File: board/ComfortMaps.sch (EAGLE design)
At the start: 47 parts, among them J1 PROG_HDR, J5 0545482271, J6 0545482271, U1 ADXL362, U3 ADP160-3.3, U4 MCP73833, X1 RASPI_GPIO_B+#_PIN

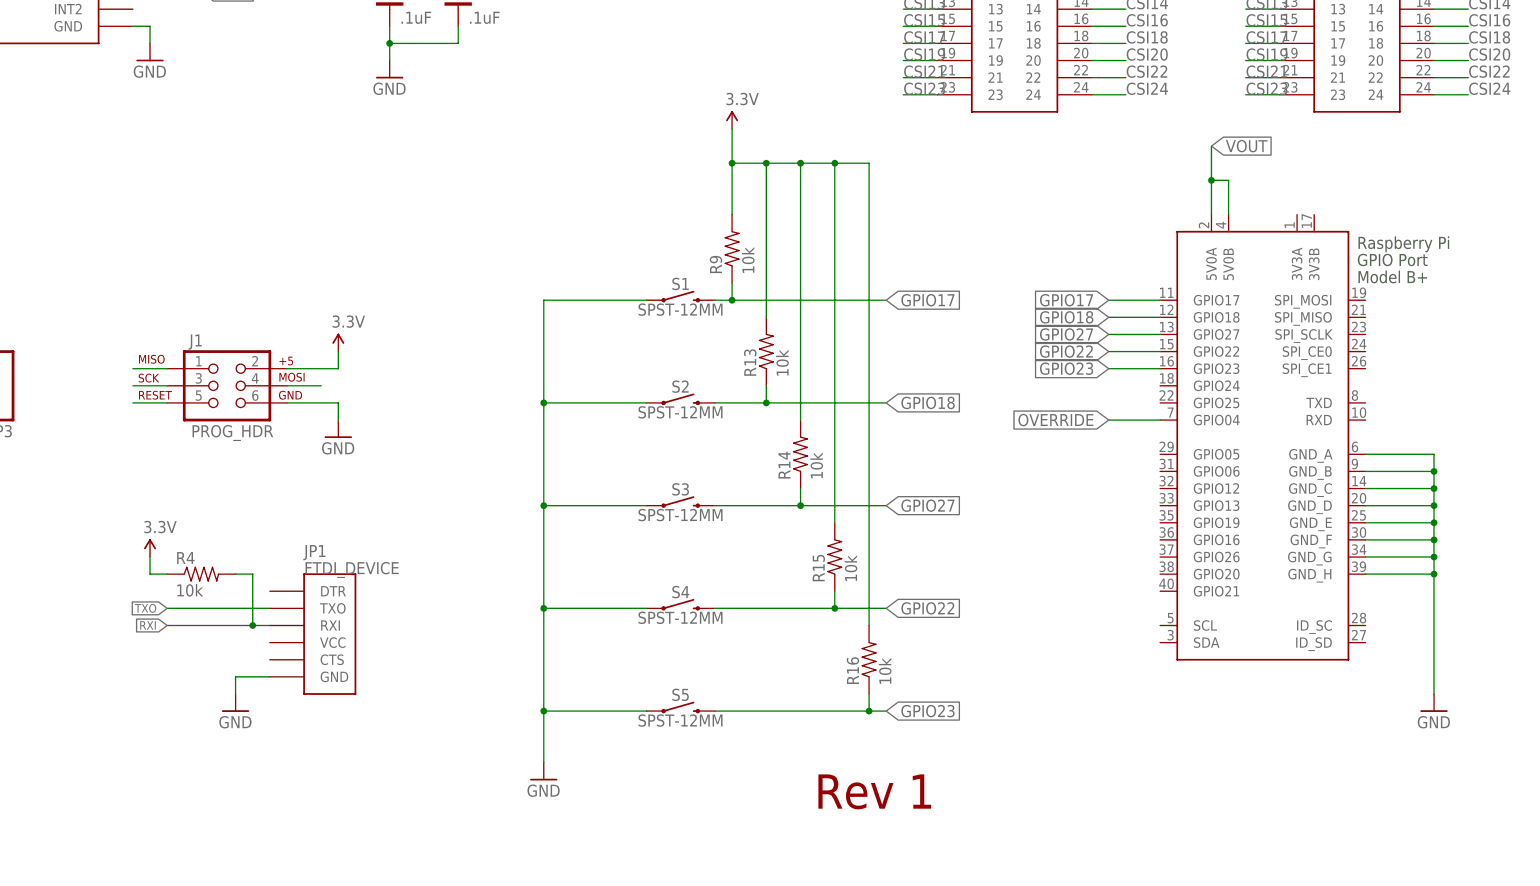
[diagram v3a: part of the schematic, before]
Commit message: Latest, before upwork.
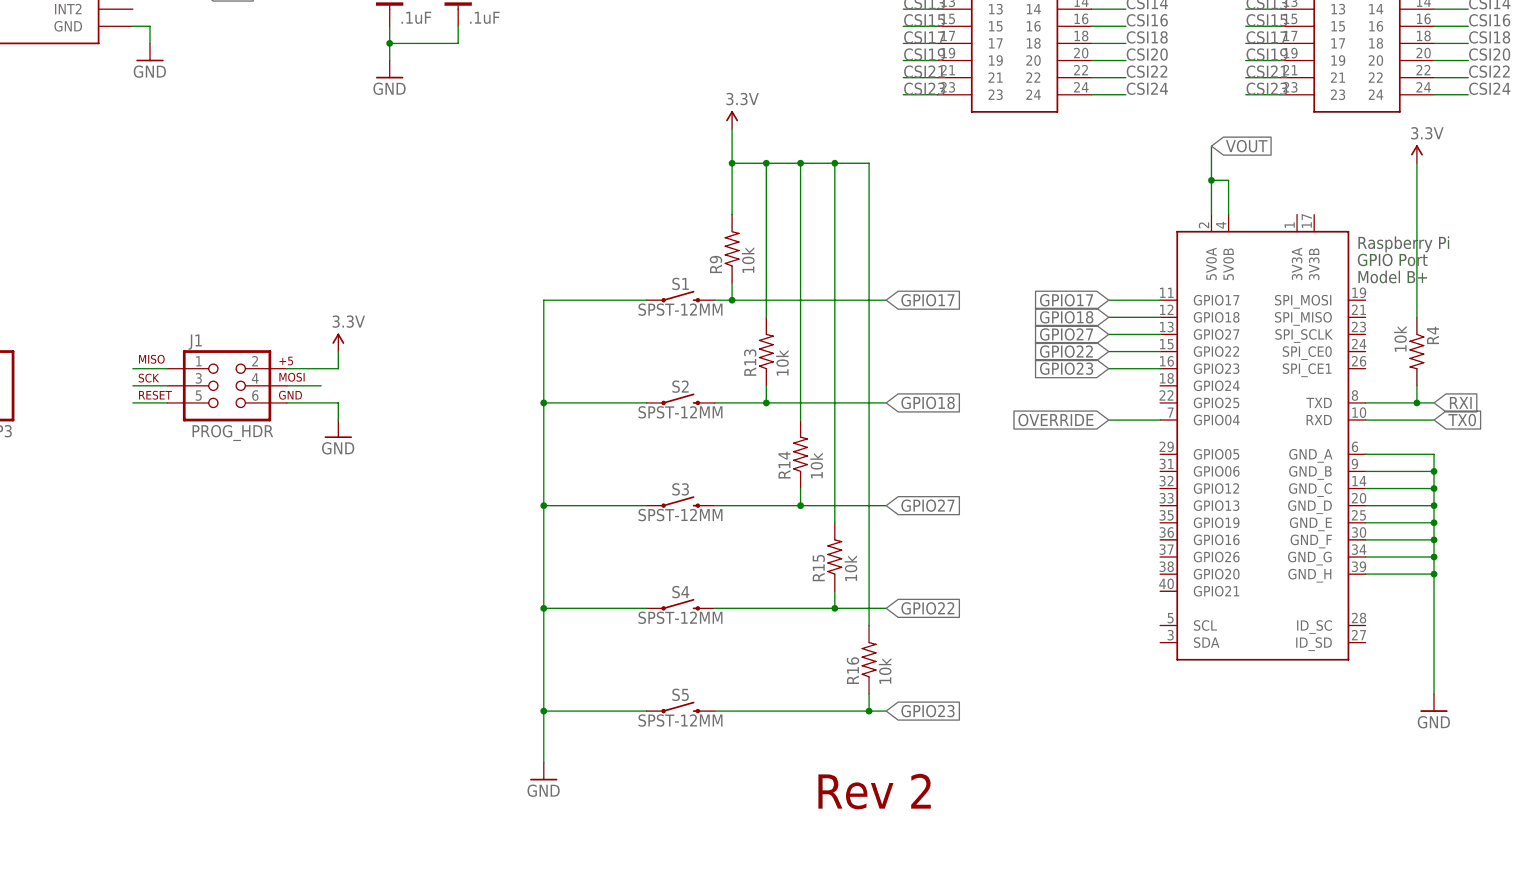
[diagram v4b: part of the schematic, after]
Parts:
- removed JP1: FTDI_DEVICE, SparkFun-Connectors:FTDI_DEVICE
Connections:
- new net TX0: X1.RXD
- net GND: no longer JP1.GND
- net RXI: now also X1.TXD; no longer JP1.RXI
- net TXO: no longer JP1.TXO
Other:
- note added: "Rev 2"
- note removed: "Rev 1"
- moved on the sheet: R4
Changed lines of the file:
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@@
 <?xml version="1.0" encoding="utf-8"?>
 <!DOCTYPE eagle SYSTEM "eagle.dtd">
-<eagle version="9.5.1">
+<eagle version="9.5.2">
 <drawing>
 <settings>
@@
 </part>
 <part name="JP3" library="SparkFun-Connectors" deviceset="M03" device="PTH"/>
-<part name="JP1" library="SparkFun-Connectors" deviceset="FTDI_DEVICE" device=""/>
 <part name="D2" library="SparkFun-DiscreteSemi" deviceset="DIODE-SCHOTTKY" device="" value="RB751">
 <attribute name="PROD_ID" value="DIO-11018"/>
@@
 </part>
 <part name="P+6" library="SparkFun-Aesthetics" deviceset="3.3V" device=""/>
-<part name="GND7" library="SparkFun-Aesthetics" deviceset="GND" device=""/>
 <part name="R4" library="SparkFun-Resistors" deviceset="10K-1%" device="RES-00824" value="10k">
 <attribute name="PROD_ID" value="RES-00824"/>
@@
 <sheet>
 <plain>
-<text x="238.252" y="5.842" size="5.08" layer="94">Rev 1</text>
+<text x="238.252" y="5.842" size="5.08" layer="94">Rev 2</text>
 <text x="2.54" y="2.54" size="1.778" layer="94">Original wake-on-shake concept by
 Nitzan Gadish, Analog Devices</text>
@@
 <attribute name="NAME" x="119.38" y="62.738" size="1.778" layer="95" rot="R180"/>
 </instance>
-<instance part="JP1" gate="G$1" x="162.56" y="33.02" smashed="yes">
-<attribute name="NAME" x="162.56" y="43.18" size="1.778" layer="95"/>
-<attribute name="VALUE" x="162.56" y="40.64" size="1.778" layer="96"/>
-</instance>
 <instance part="D2" gate="G$1" x="66.04" y="45.72" smashed="yes">
 <attribute name="PROD_ID" x="66.04" y="45.72" size="1.778" layer="96" display="off"/>
@@
 <attribute name="VALUE" x="16.764" y="140.716" size="1.778" layer="96"/>
 </instance>
-<instance part="GND7" gate="1" x="152.4" y="20.32" smashed="yes">
-<attribute name="VALUE" x="149.86" y="17.78" size="1.778" layer="96"/>
-</instance>
-<instance part="R4" gate="G$1" x="147.32" y="40.64" smashed="yes">
-<attribute name="PROD_ID" x="147.32" y="40.64" size="1.778" layer="96" display="off"/>
-<attribute name="NAME" x="143.51" y="42.1386" size="1.778" layer="95"/>
-<attribute name="VALUE" x="143.51" y="37.338" size="1.778" layer="96"/>
-</instance>
-<instance part="P+7" gate="G$1" x="139.7" y="43.18" smashed="yes">
-<attribute name="VALUE" x="138.684" y="46.736" size="1.778" layer="96"/>
+<instance part="R4" gate="G$1" x="327.66" y="73.66" smashed="yes" rot="R270">
+<attribute name="PROD_ID" x="327.66" y="73.66" size="1.778" layer="96" rot="R270" display="off"/>
+<attribute name="NAME" x="329.1586" y="77.47" size="1.778" layer="95" rot="R270"/>
+<attribute name="VALUE" x="324.358" y="77.47" size="1.778" layer="96" rot="R270"/>
+</instance>
+<instance part="P+7" gate="G$1" x="327.66" y="101.6" smashed="yes">
+<attribute name="VALUE" x="326.644" y="105.156" size="1.778" layer="96"/>
 </instance>
 <instance part="S1" gate="G$1" x="218.44" y="81.28" smashed="yes">
@@
 <pinref part="GND6" gate="1" pin="GND"/>
 <wire x1="167.64" y1="66.04" x2="167.64" y2="63.5" width="0.1524" layer="91"/>
-</segment>
-<segment>
-<pinref part="JP1" gate="G$1" pin="GND"/>
-<wire x1="157.48" y1="25.4" x2="152.4" y2="25.4" width="0.1524" layer="91"/>
-<wire x1="152.4" y1="25.4" x2="152.4" y2="22.86" width="0.1524" layer="91"/>
-<pinref part="GND7" gate="1" pin="GND"/>
 </segment>
 <segment>
@@
 <segment>
 <pinref part="P+7" gate="G$1" pin="3.3V"/>
-<wire x1="139.7" y1="43.18" x2="139.7" y2="40.64" width="0.1524" layer="91"/>
+<wire x1="327.66" y1="101.6" x2="327.66" y2="78.74" width="0.1524" layer="91"/>
 <pinref part="R4" gate="G$1" pin="1"/>
-<wire x1="139.7" y1="40.64" x2="142.24" y2="40.64" width="0.1524" layer="91"/>
 </segment>
 <segment>
@@
 </segment>
 <segment>
-<pinref part="JP1" gate="G$1" pin="RXI"/>
-<wire x1="157.48" y1="33.02" x2="154.94" y2="33.02" width="0.1524" layer="91"/>
-<label x="142.24" y="33.02" size="1.27" layer="95" rot="R180" xref="yes"/>
+<pinref part="X1" gate="G$1" pin="TXD"/>
+<wire x1="320.04" y1="66.04" x2="327.66" y2="66.04" width="0.1524" layer="91"/>
+<label x="330.2" y="66.04" size="1.778" layer="95" xref="yes"/>
 <pinref part="R4" gate="G$1" pin="2"/>
-<wire x1="154.94" y1="33.02" x2="142.24" y2="33.02" width="0.1524" layer="91"/>
-<wire x1="152.4" y1="40.64" x2="154.94" y2="40.64" width="0.1524" layer="91"/>
-<wire x1="154.94" y1="40.64" x2="154.94" y2="33.02" width="0.1524" layer="91"/>
-<junction x="154.94" y="33.02"/>
+<wire x1="327.66" y1="66.04" x2="330.2" y2="66.04" width="0.1524" layer="91"/>
+<wire x1="327.66" y1="68.58" x2="327.66" y2="66.04" width="0.1524" layer="91"/>
+<junction x="327.66" y="66.04"/>
 </segment>
 </net>
@@
 <wire x1="33.02" y1="129.54" x2="25.4" y2="129.54" width="0.1524" layer="91"/>
 <label x="25.4" y="129.54" size="1.27" layer="95" rot="R180" xref="yes"/>
-</segment>
-<segment>
-<pinref part="JP1" gate="G$1" pin="TXO"/>
-<wire x1="157.48" y1="35.56" x2="142.24" y2="35.56" width="0.1524" layer="91"/>
-<label x="142.24" y="35.56" size="1.27" layer="95" rot="R180" xref="yes"/>
 </segment>
 </net>
@@
 </segment>
 </net>
+<net name="TX0" class="0">
+<segment>
+<pinref part="X1" gate="G$1" pin="RXD"/>
+<wire x1="320.04" y1="63.5" x2="330.2" y2="63.5" width="0.1524" layer="91"/>
+<label x="330.2" y="63.5" size="1.778" layer="95" xref="yes"/>
+</segment>
+</net>
